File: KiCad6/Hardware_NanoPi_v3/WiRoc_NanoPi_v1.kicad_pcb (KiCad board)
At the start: 2 copper layers, 43.8 x 68.3 mm, 134 parts, among them J1 Conn_01x02, J2 USB_Power_02x02, J3 JST-2PIN, J4 USB_Host_Data_02x02, J5 Conn_01x03, J6 HAT_Conn_DBG, J7 NanoPIAir, J8 USB_Host_Data_02x02, J9 Conn_Coaxial, SW1 SW_SPST, U1 DRF1268DS, U2 OLED, U3 AXP209, U4 LP6226_SY7208, U5 SY6280, U6 BatteryPadM, U7 BatteryPadP

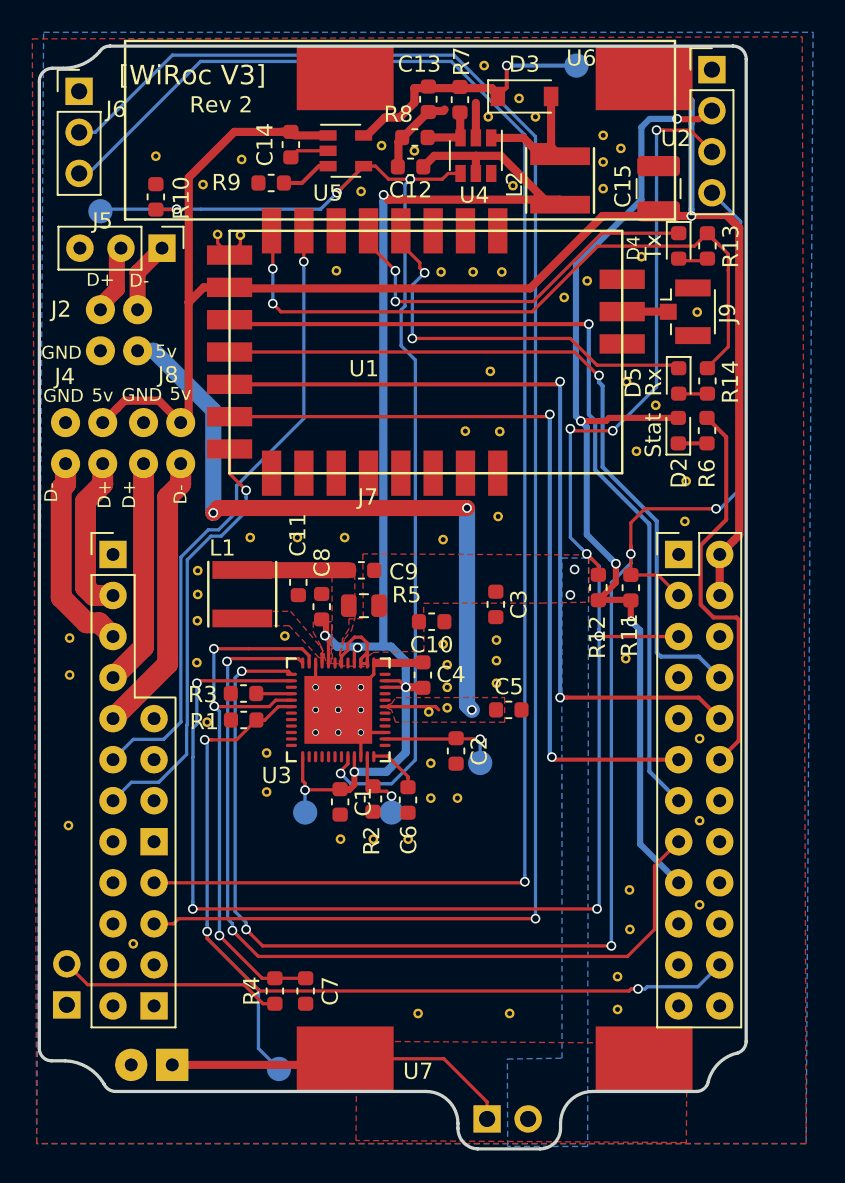
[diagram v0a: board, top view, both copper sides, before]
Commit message: diverse SRR etc
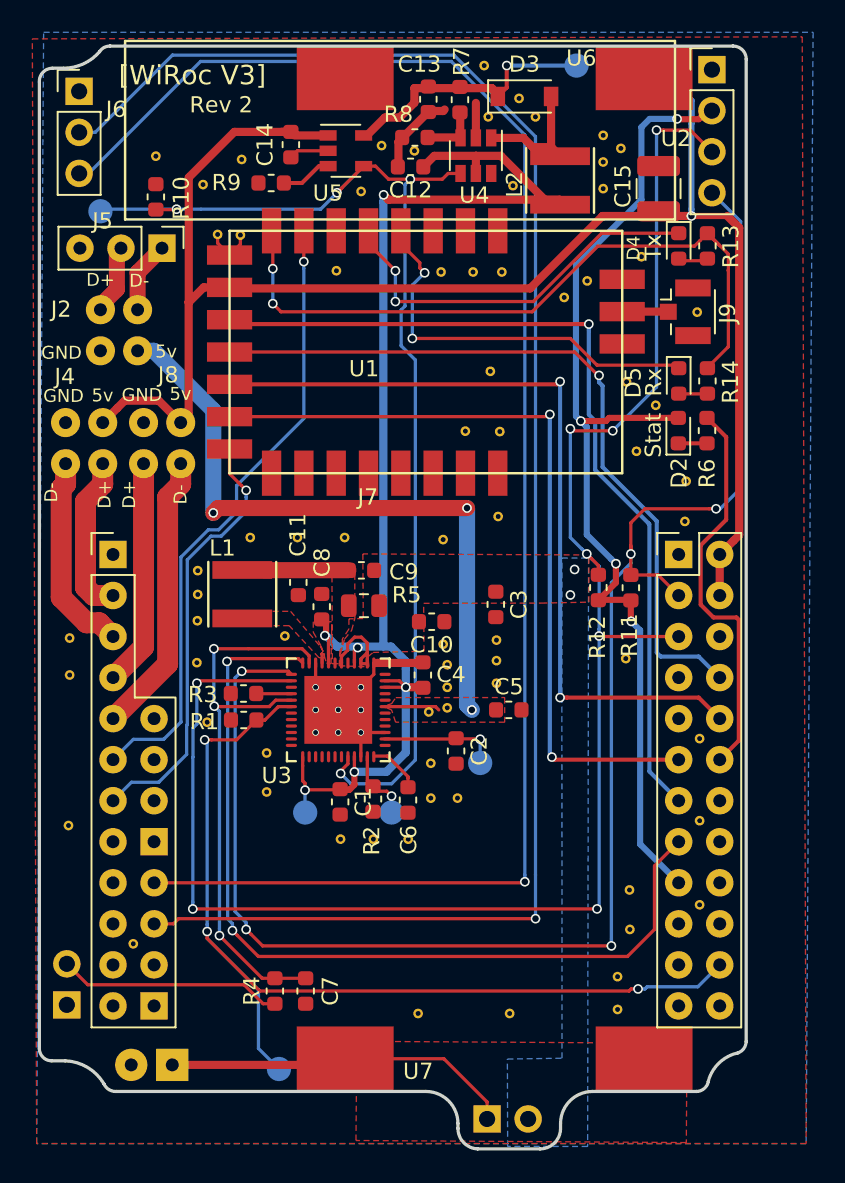
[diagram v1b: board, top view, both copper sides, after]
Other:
- net class Default removed
- net class Power removed
- net class Signal removed
